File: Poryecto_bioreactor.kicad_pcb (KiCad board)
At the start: 2 copper layers, 35 parts, among them J1 Screw_Terminal_01x02, Q1 IRLZ44N, Q2 BSS138, U2 OKI-78SR-5/1.5-W36-C (L7805)

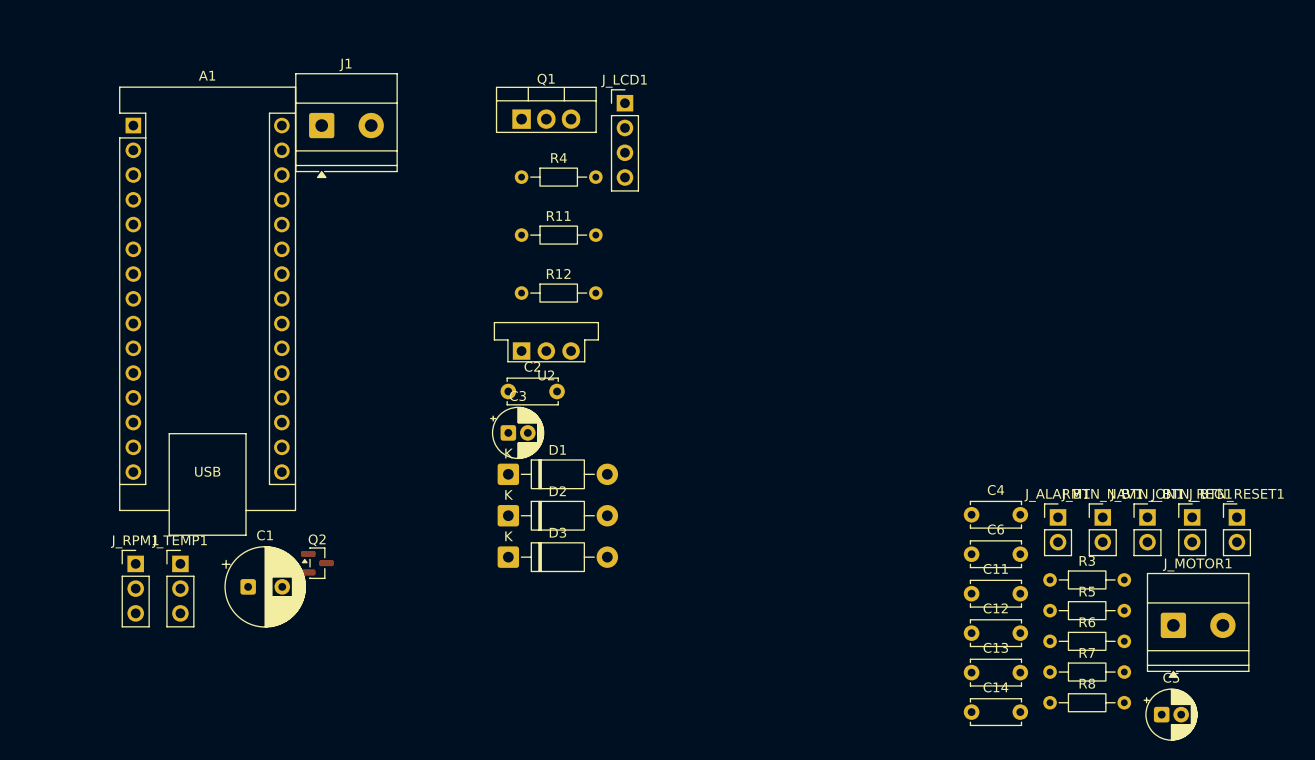
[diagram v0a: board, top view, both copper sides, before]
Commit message: pcb_act
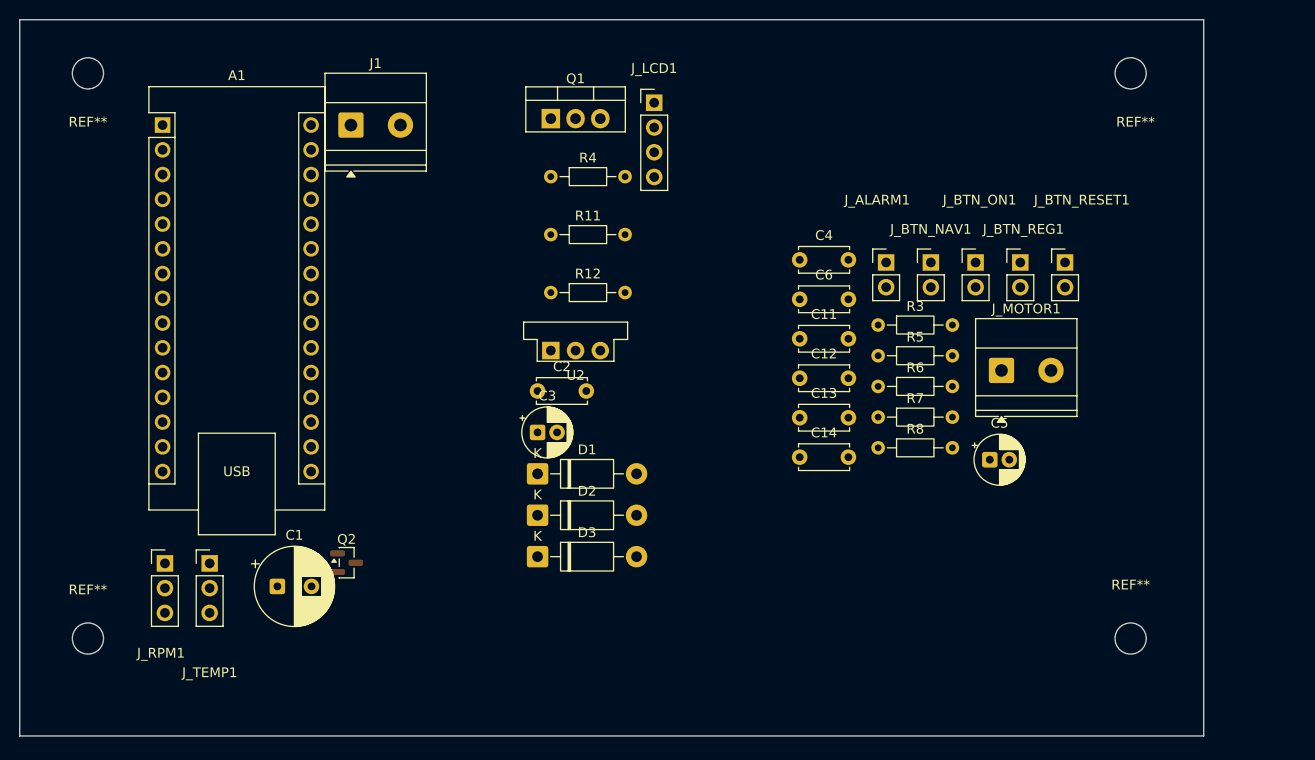
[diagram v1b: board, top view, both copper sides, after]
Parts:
- added REF**: MountingHole_3.2mm_M3, MountingHole:MountingHole_3.2mm_M3, F.Cu at (130.0, 19.0)
- added REF**: MountingHole_3.2mm_M3, MountingHole:MountingHole_3.2mm_M3, F.Cu at (130.0, 76.5)
- added REF**: MountingHole_3.2mm_M3, MountingHole:MountingHole_3.2mm_M3, F.Cu at (23.0, 19.0)
- added REF**: MountingHole_3.2mm_M3, MountingHole:MountingHole_3.2mm_M3, F.Cu at (22.5, 77.0)
- moved C11 31.6 mm to (96.0, 46.2)
- moved C12 31.6 mm to (96.0, 50.3)
- moved C5 31.6 mm to (115.5, 58.6)
- moved R5 31.6 mm to (104.1, 48.0)
- moved R6 31.6 mm to (104.1, 51.1)
- moved R8 31.6 mm to (104.1, 57.4)
- moved C13 31.6 mm to (96.0, 54.3)
- moved C14 31.6 mm to (96.0, 58.4)
- moved C4 31.6 mm to (96.0, 38.1)
- moved C6 31.6 mm to (96.0, 42.2)
- moved J_ALARM1 31.6 mm to (104.9, 38.4)
- moved J_BTN_NAV1 31.6 mm to (109.5, 38.4)
- moved J_BTN_RESET1 31.6 mm to (123.3, 38.4)
- moved R3 31.6 mm to (104.1, 44.8)
- moved R7 31.6 mm to (104.1, 54.3)
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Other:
- board outline added: 121.5 x 73.5 mm
